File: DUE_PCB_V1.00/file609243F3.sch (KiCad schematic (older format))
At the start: 20 parts, among them J26 Motor Left, J27 Cutter Motor, J28 Motor Right, U1 MC33926, U2 MC33926

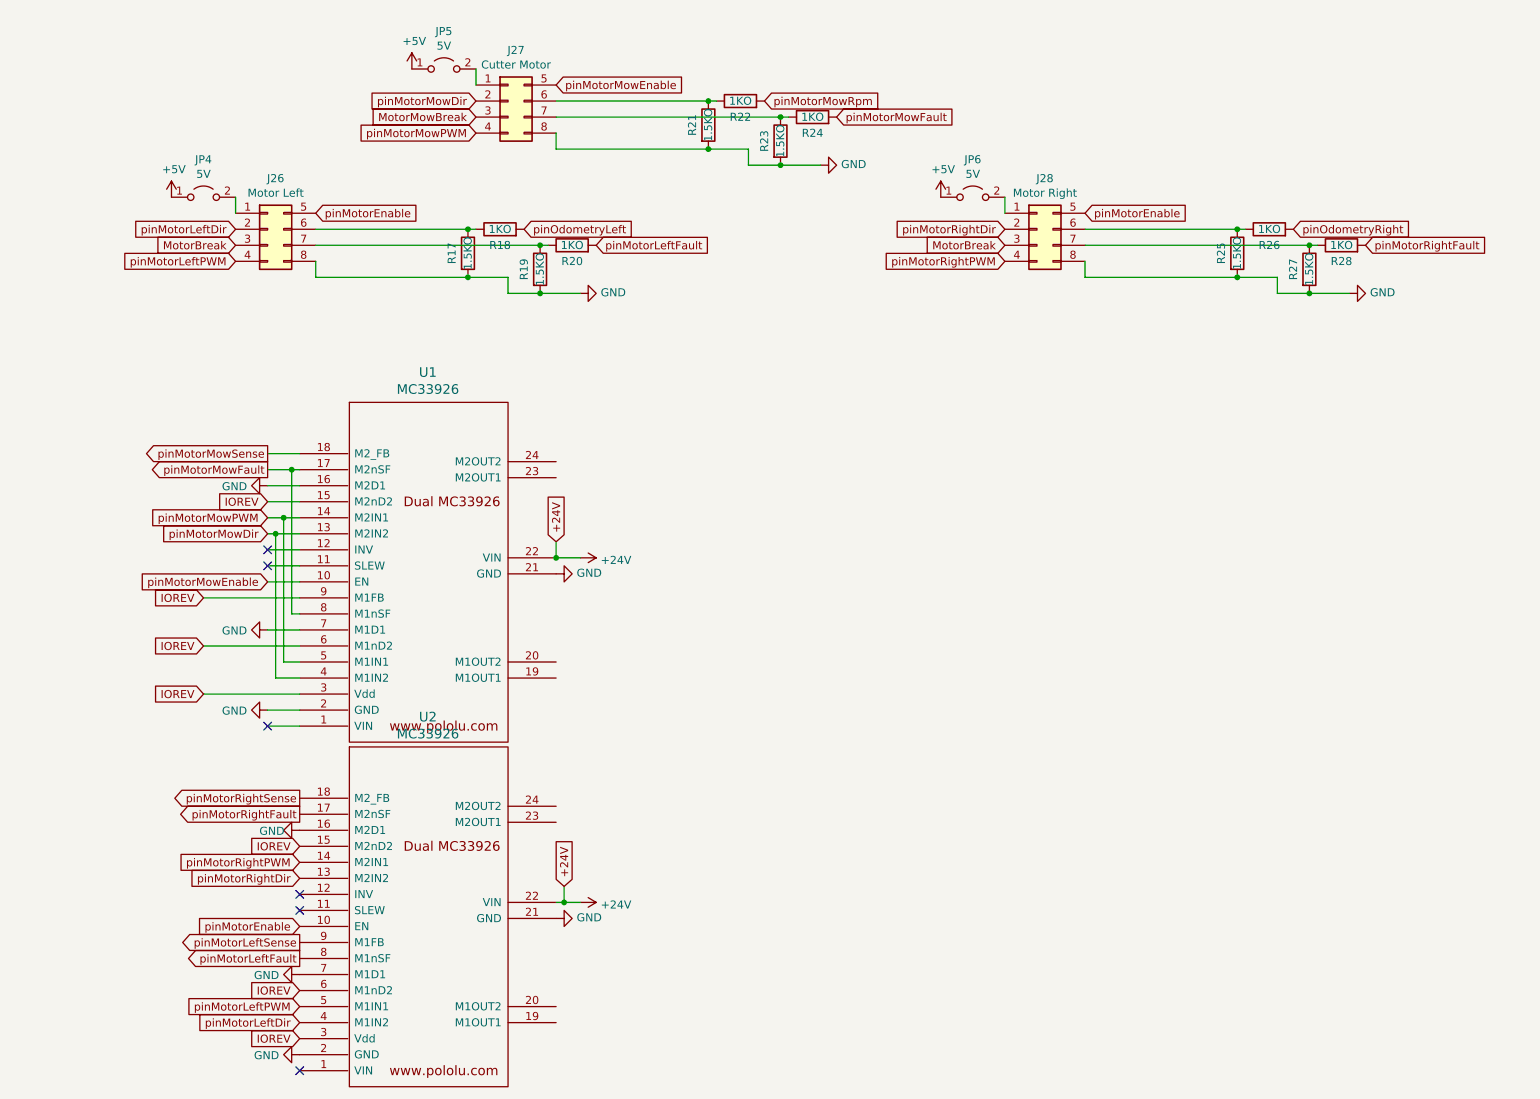
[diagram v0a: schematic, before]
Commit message: Remove 2x4 Motor Pin Connectors
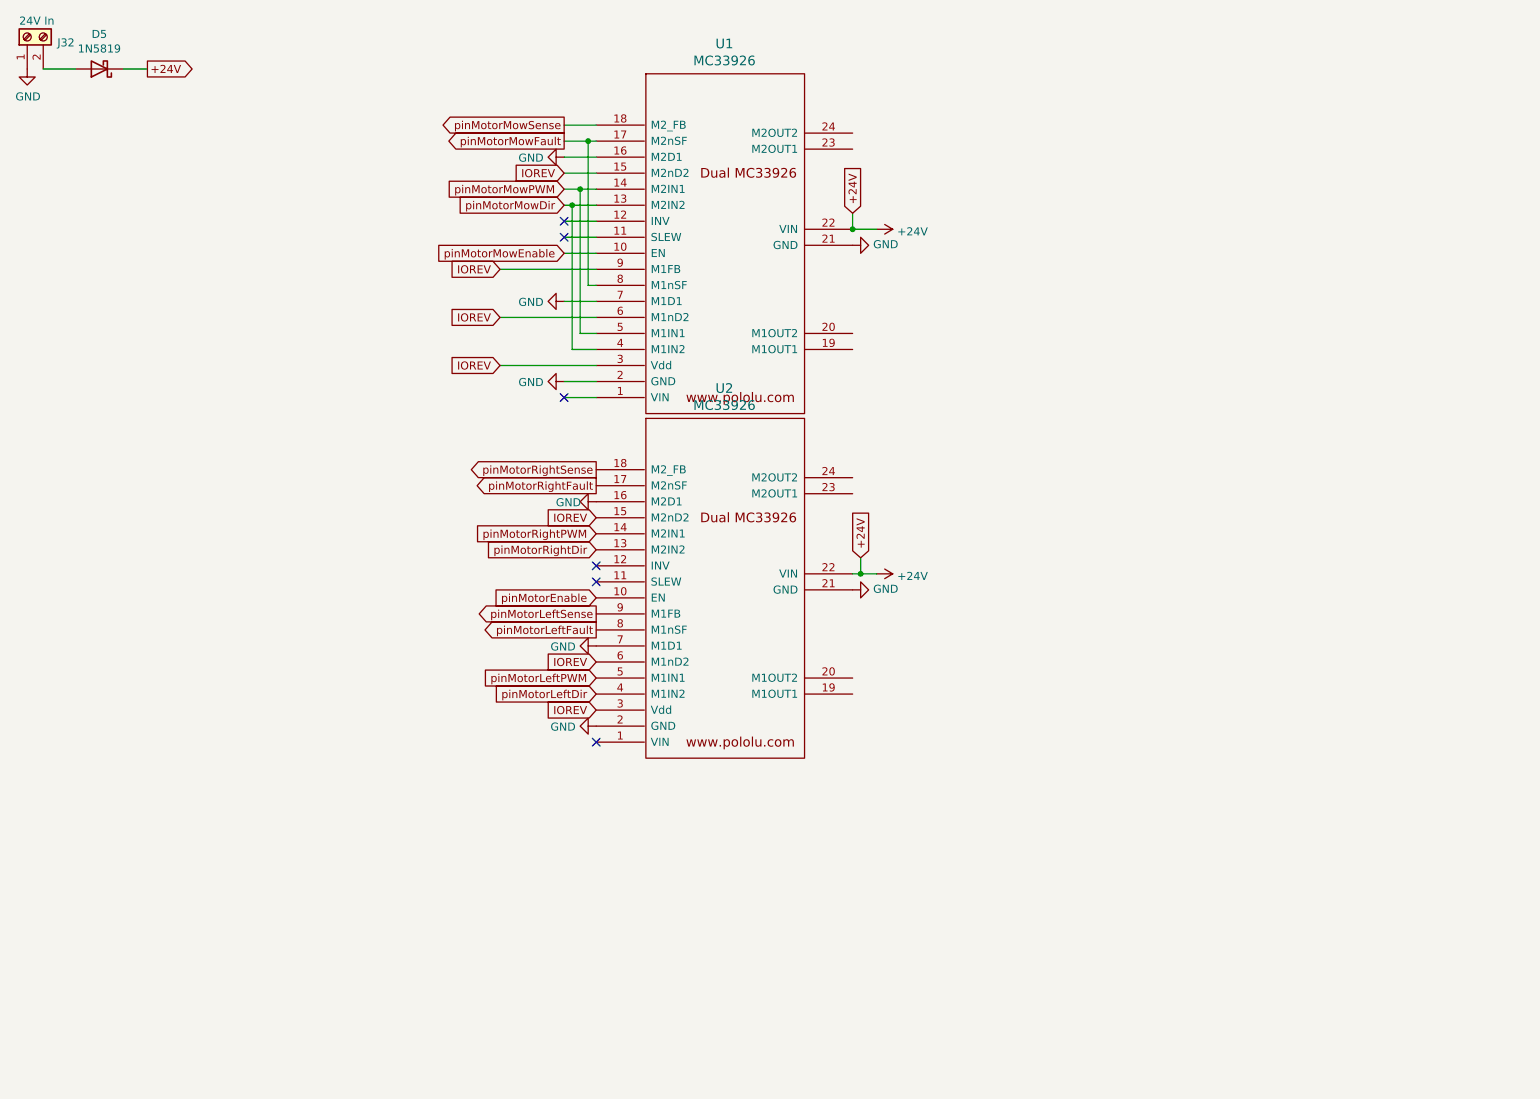
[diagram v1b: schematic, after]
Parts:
- removed J26: Motor Left, Connector_PinSocket_2.54mm:PinSocket_2x04_P2.54mm_Vertical, symbol Connector_Generic:Conn_02x04_Top_Bottom
- removed J27: Cutter Motor, Connector_PinSocket_2.54mm:PinSocket_2x04_P2.54mm_Vertical, symbol Connector_Generic:Conn_02x04_Top_Bottom
- removed J28: Motor Right, Connector_PinSocket_2.54mm:PinSocket_2x04_P2.54mm_Vertical, symbol Connector_Generic:Conn_02x04_Top_Bottom
- removed JP4, JP5, JP6: 5V, Connector_PinSocket_2.54mm:PinSocket_1x02_P2.54mm_Vertical, symbol Jumper:Jumper_2_Open
- removed R17, R19, R21, R23, R25, R27: 1.5KO, Resistor_THT:R_Axial_DIN0207_L6.3mm_D2.5mm_P2.54mm_Vertical, symbol Device:R
- removed R18, R20, R22, R24, R26, R28: 1KO, Resistor_THT:R_Axial_DIN0207_L6.3mm_D2.5mm_P2.54mm_Vertical, symbol Device:R
- added D5: 1N5819, Diode_THT:D_DO-41_SOD81_P10.16mm_Horizontal, symbol Diode:1N5819
- added J32: 24V In, TerminalBlock:TerminalBlock_bornier-2_P5.08mm, symbol Connector:Screw_Terminal_01x02
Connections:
- net +24V: now also D5.1 (K)
- net GND: now also J32.1 (Pin_1)
- new net: D5.2 (A), J32.2 (Pin_2)
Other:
- moved on the sheet: U1, U2
